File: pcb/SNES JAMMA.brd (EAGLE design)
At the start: 66 x 63.5 mm, 10 parts, among them P1-JAMMA-A PLAYER 1 JAMMA, P2-JAMMA-A PLAYER 2 JAMMA

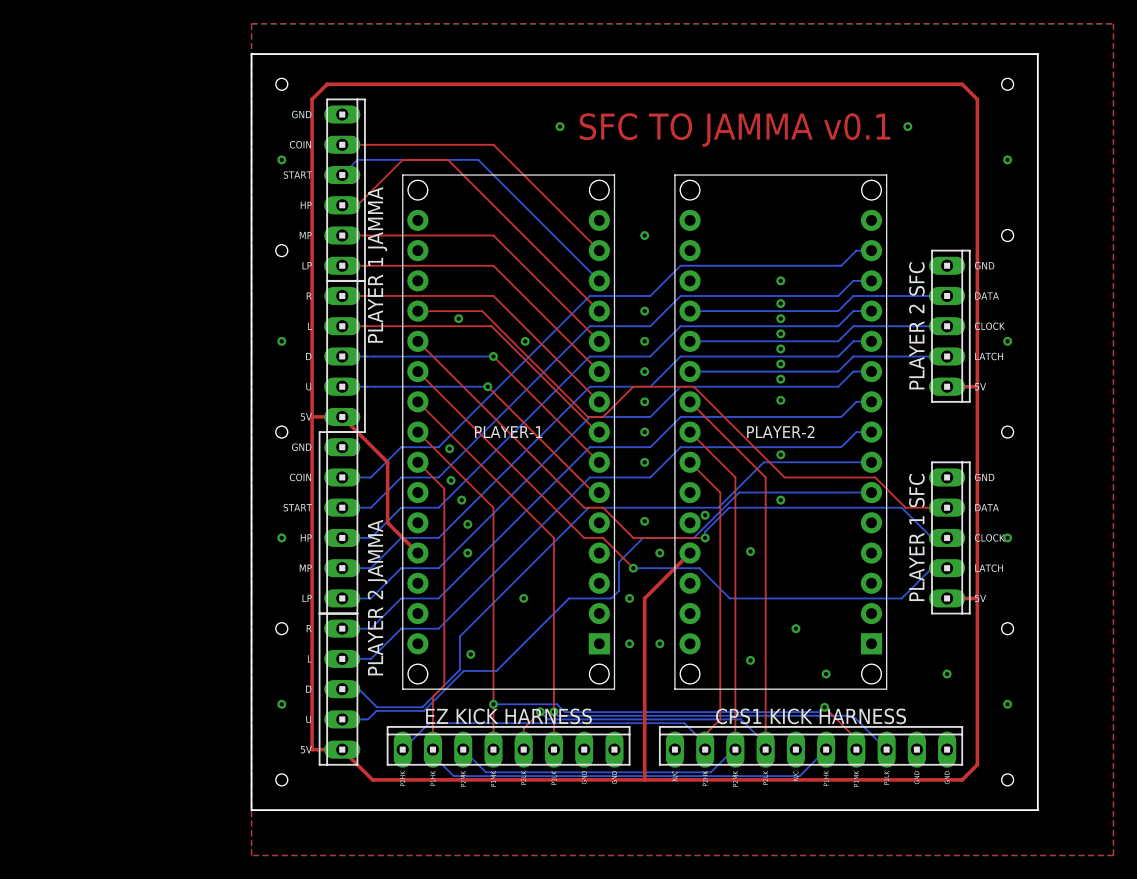
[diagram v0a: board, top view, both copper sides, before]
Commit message: v1.0 PCB and Schematics files
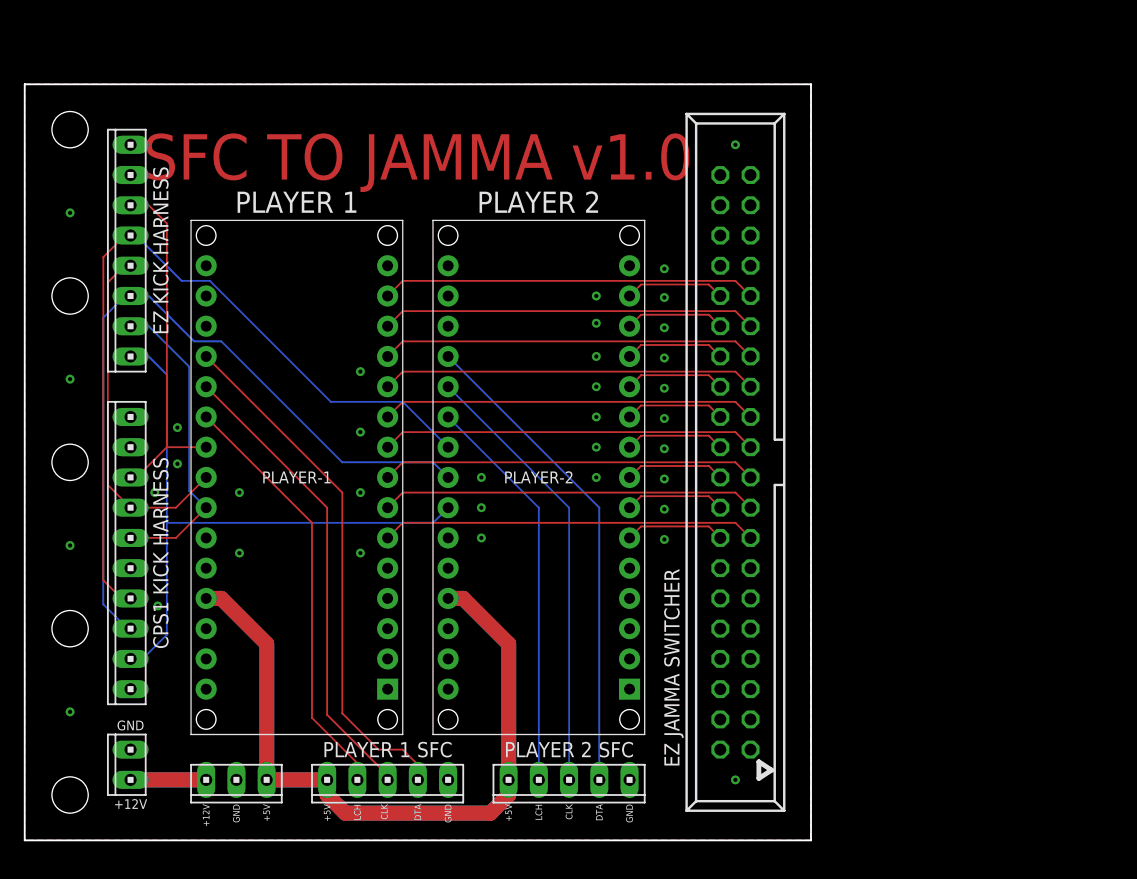
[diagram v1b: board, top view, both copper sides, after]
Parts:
- removed P1-JAMMA-A: PLAYER 1 JAMMA, con-amp:10X05MTA
- removed P1-JAMMA-B, P2-JAMMA-B: (no value), con-amp:10X06MTA
- removed P2-JAMMA-A: PLAYER 2 JAMMA, con-amp:10X05MTA
- added J1: 12V POWER, con-amp:10X02MTA
- added J2: (no value), con-amp:10X03MTA
- added JAMMA: 057-040-1, con-panduit:057-040-1
- moved CPS1-KICK 59.5 mm to (8.89, 24.1), turned to 90 degrees
- moved EZ-KICK 52.6 mm to (8.89, 49.5), turned to 90 degrees
- moved SFC-PLAYER-1 51.2 mm to (30.5, 5.08), turned to 180 degrees
- moved SFC-PLAYER-2 49.6 mm to (45.7, 5.08), turned to 180 degrees
- moved PLAYER-2 20.7 mm to (43.2, 30.5)
- moved PLAYER-1 18.2 mm to (22.9, 30.5)
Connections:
- net P1-H-KICK renamed P1-BTN6
- net P1-L-KICK renamed P1-BTN4
- net P1-M-KICK renamed P1-BTN5
- net P2-H-KICK renamed P2-BTN6
- net P2-L-KICK renamed P2-BTN4
- net P2-M-KICK renamed P2-BTN5
- removed net P1-JAMMA-COIN: P1-JAMMA-B.5, PLAYER-1.J1.14
- removed net P1-JAMMA-DOWN: P1-JAMMA-A.3, PLAYER-1.J1.7
- removed net P1-JAMMA-H-PUNCH: P1-JAMMA-B.3, PLAYER-1.J1.12
- removed net P1-JAMMA-L-PUNCH: P1-JAMMA-B.1, PLAYER-1.J1.10
- removed net P1-JAMMA-LEFT: P1-JAMMA-A.4, PLAYER-1.J1.8
- removed net P1-JAMMA-M-PUNCH: P1-JAMMA-B.2, PLAYER-1.J1.11
- removed net P1-JAMMA-RIGHT: P1-JAMMA-A.5, PLAYER-1.J1.9
- removed net P1-JAMMA-START: P1-JAMMA-B.4, PLAYER-1.J1.13
- removed net P1-JAMMA-UP: P1-JAMMA-A.2, PLAYER-1.J1.6
- removed net P2-JAMMA-COIN: P2-JAMMA-B.2, PLAYER-2.J1.14
- removed net P2-JAMMA-DOWN: P2-JAMMA-A.3, PLAYER-2.J1.7
- removed net P2-JAMMA-H-PUNCH: P2-JAMMA-B.4, PLAYER-2.J1.12
- removed net P2-JAMMA-L-PUNCH: P2-JAMMA-B.6, PLAYER-2.J1.10
- removed net P2-JAMMA-LEFT: P2-JAMMA-A.2, PLAYER-2.J1.8
- removed net P2-JAMMA-M-PUNCH: P2-JAMMA-B.5, PLAYER-2.J1.11
- removed net P2-JAMMA-RIGHT: P2-JAMMA-A.1, PLAYER-2.J1.9
- removed net P2-JAMMA-START: P2-JAMMA-B.3, PLAYER-2.J1.13
- removed net P2-JAMMA-UP: P2-JAMMA-A.4, PLAYER-2.J1.6
- new net +12V: J1.2, J2.1
- new net N$6: PLAYER-1.J1.15
- new net P1-BTN1: JAMMA.27, PLAYER-1.J1.12
- new net P1-BTN2: JAMMA.29, PLAYER-1.J1.13
- new net P1-BTN3: JAMMA.31, PLAYER-1.J1.14
- new net P1-COIN: JAMMA.15, PLAYER-1.J1.6
- new net P1-DOWN: JAMMA.21, PLAYER-1.J1.9
- new net P1-LEFT: JAMMA.23, PLAYER-1.J1.10
- new net P1-RIGHT: JAMMA.25, PLAYER-1.J1.11
- new net P1-START: JAMMA.17, PLAYER-1.J1.7
- new net P1-UP: JAMMA.19, PLAYER-1.J1.8
- new net P2-BTN1: JAMMA.28, PLAYER-2.J1.12
- new net P2-BTN2: JAMMA.30, PLAYER-2.J1.13
- new net P2-BTN3: JAMMA.32, PLAYER-2.J1.14
- new net P2-COIN: JAMMA.16, PLAYER-2.J1.6
- new net P2-DOWN: JAMMA.22, PLAYER-2.J1.9
- new net P2-LEFT: JAMMA.24, PLAYER-2.J1.10
- new net P2-RIGHT: JAMMA.26, PLAYER-2.J1.11
- new net P2-START: JAMMA.18, PLAYER-2.J1.7
- new net P2-UP: JAMMA.20, PLAYER-2.J1.8
- net GND: now also J1.1, J2.2; no longer P1-JAMMA-B.6, P2-JAMMA-B.1
- net VCC: now also J2.3; no longer P1-JAMMA-A.1, P2-JAMMA-A.5
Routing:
- net VCC: track 267.2 -> 120.6 mm
- net P2-JAMMA-DOWN: track 55.2 -> 0.00 mm
- net P2-JAMMA-UP: track 53.8 -> 0.00 mm
- net P2-JAMMA-LEFT: track 52.3 -> 0.00 mm
- net P2-JAMMA-COIN: track 52.3 -> 0.00 mm
- net P2-JAMMA-H-PUNCH: track 52.3 -> 0.00 mm
- net P2-JAMMA-START: track 52.3 -> 0.00 mm
- net P2-JAMMA-RIGHT: track 52.3 -> 0.00 mm
- net P2-JAMMA-M-PUNCH: track 52.3 -> 0.00 mm
- net P2-JAMMA-L-PUNCH: track 52.3 -> 0.00 mm
- net P1-BTN6: track 60.6 -> 26.2 mm
- net P1-BTN4: track 63.2 -> 29.9 mm, vias 1 -> 0
- net P1-BTN5: track 62.2 -> 29.6 mm, vias 2 -> 0
- net P1-COIN: track 0.00 -> 31.5 mm
- net P1-BTN3: track 0.00 -> 31.5 mm
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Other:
- board text added: "+12V"
- board text added: "+5V"
- board text added: "CLK"
- board text added: "DTA"
- board text added: "EZ JAMMA SWITCHER"
- board text added: "LCH"
- board text added: "PLAYER 1"
- board text added: "PLAYER 2"
- board text added: "SFC TO JAMMA v1.0"
- board text removed: "5V"
- board text removed: "CLOCK"
- board text removed: "COIN"
- board text removed: "D"
- board text removed: "DATA"
- board text removed: "HP"
- board text removed: "L"
- board text removed: "LATCH"
- board text removed: "LP"
- board text removed: "MP"
- board text removed: "N/C"
- board text removed: "P1HK"
- board text removed: "P1LK"
- board text removed: "P1MK"
- board text removed: "P2HK"
- board text removed: "P2LK"
- board text removed: "P2MK"
- board text removed: "R"
- board text removed: "SFC TO JAMMA v0.1"
- board text removed: "START"
- board text removed: "U"
